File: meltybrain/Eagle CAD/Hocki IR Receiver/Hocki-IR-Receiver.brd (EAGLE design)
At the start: 160 x 100 mm, 0 parts

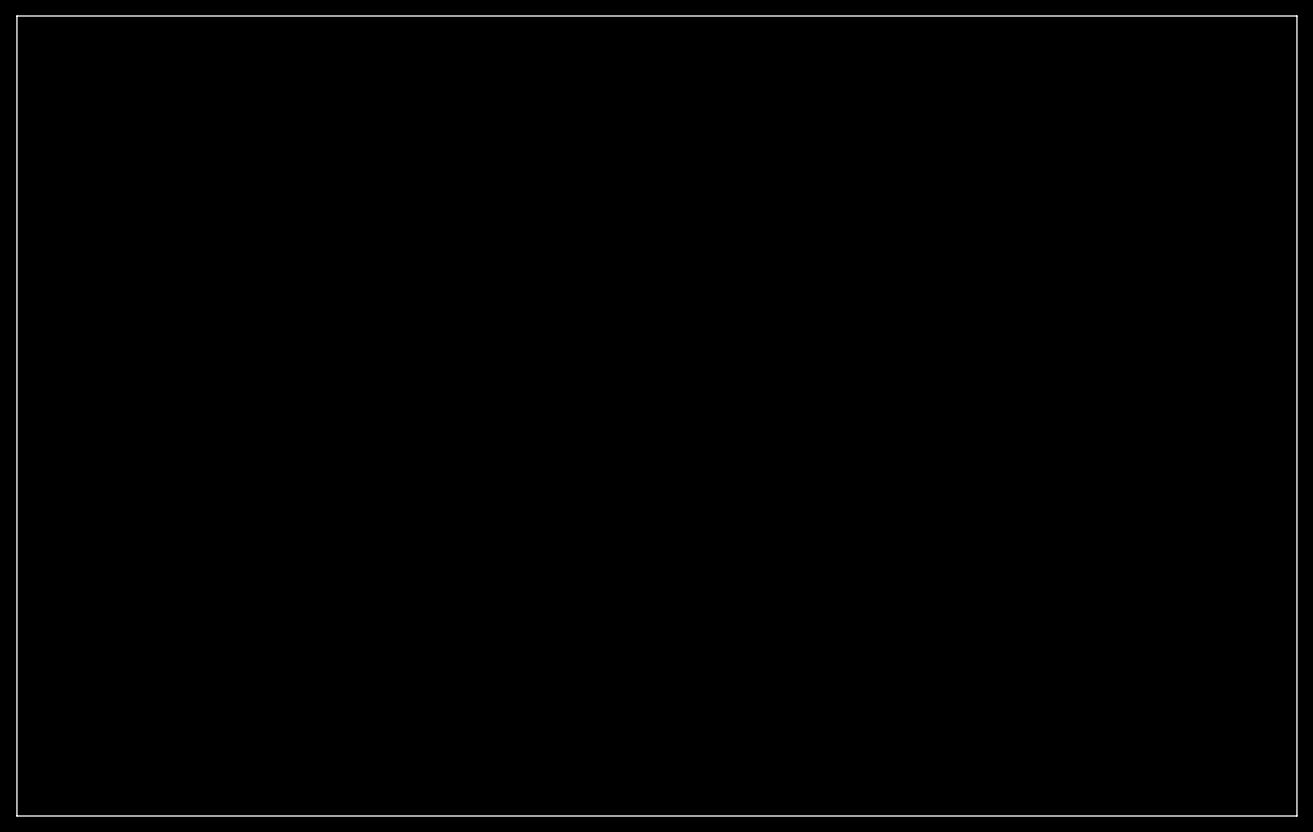
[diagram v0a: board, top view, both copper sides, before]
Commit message: broke something. this is a test
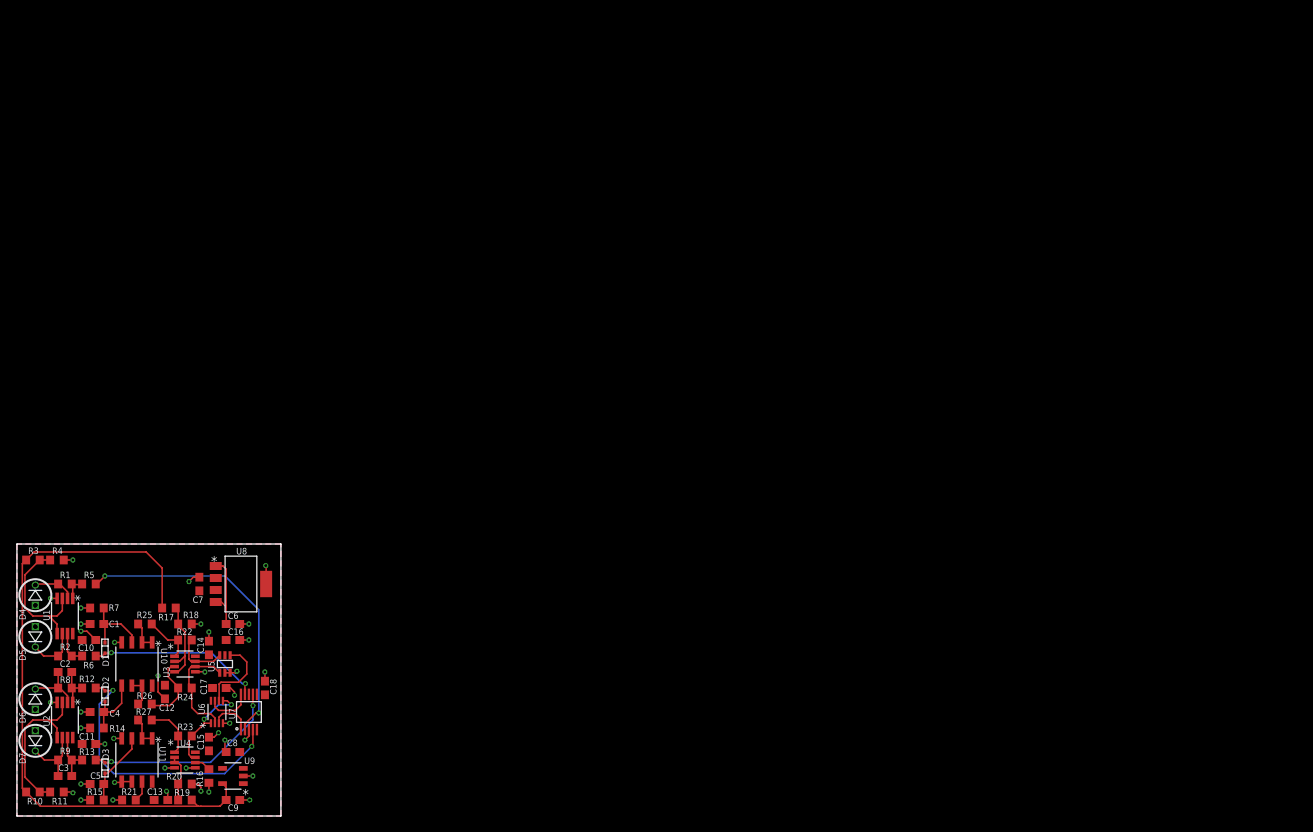
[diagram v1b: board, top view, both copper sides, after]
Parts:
- added C1, C4, C5: 50n, rcl:C0603
- added C10, C11, C6, C7, C8, C9: 1u, rcl:C0603
- added C12, C13, C14, C15, C16, C17, C18: 0.1u, rcl:C0603
- added C2: 0.5p, rcl:C0603
- added C3: 2p, rcl:C0603
- added D1, D2, D3: RB521S30T1G, Hocki_library:SOD-523
- added D4, D5, D6, D7: TEFD4300F, Hocki_library:TEFD4300F
- added R1: 10M, resistor:R0603
- added R10, R11, R16, R18, R20, R21, R22, R23, R24, R3, R4, R9: 10k, resistor:R0603
- added R12, R13, R5, R6: 50, resistor:R0603
- added R14, R15, R7: 30k, resistor:R0603
- added R17, R19: 3.33k, resistor:R0603
- added R2: 1M, resistor:R0603
- added R25, R26, R27: 30, resistor:R0603
- added R8: 100k, resistor:R0603
- added U1, U2: OPA2380AIDGKR, Hocki_library:8-VSSOP
- added U10, U11: LMH6612MAX/NOPB, Hocki_library:8-SOIC
- added U3, U4: TLV3502AIDCNR, Hocki_library:SOT-23-8
- added U5: SN74LVC1G58DCKR, Hocki_library:SC-70-6
- added U6: NL27WZ32USG, Hocki_library:US8
- added U7: TMUX1204DGSR, Hocki_library:10-VSSOP
- added U8: LP38693MP-5.0/NOPB, Hocki_library:SOT-223-5
- added U9: TLV73310PDBVT, Hocki_library:SOT-23-5
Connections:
- new net 1.0V: C9.1, R10.2, R17.2, R19.2, R3.2, U9.5
- new net 100KGAIN: D2.2, R12.2, U7.4
- new net 100KLOGIC: R24.1, U3.6, U5.1, U6.2
- new net 100KPEAK: C4.1, D2.1, R14.2, U10.5
- new net 10KGAIN: D3.2, R13.2, U7.7
- new net 10KLOGIC: R23.1, U4.7, U6.1, U6.5
- new net 10KPEAK: C5.1, D3.1, R15.2, U11.3
- new net 10MGAIN: R5.2, U7.2
- new net 1MGAIN: D1.2, R6.2, U7.9
- new net 1MLOGIC: R22.1, U3.7, U5.6
- new net 5V: C10.1, C11.1, C12.1, C13.1, C14.1, C15.1, C16.1, C17.1, C18.1, C7.1, C8.1, U1.8, U10.8, U11.8, U2.8, U3.8, U4.8, U5.5, U6.8, U7.5, U7.6, U8.3, U9.1, U9.3
- new net A0: U6.3, U7.1
- new net A1: U6.7, U7.10
- new net GND: C1.2, C10.2, C11.2, C12.2, C13.2, C14.2, C15.2, C16.2, C17.2, C18.2, C4.2, C5.2, C6.2, C7.2, C8.2, C9.2, D4.1, D5.1, D6.1, D7.1, R11.1, R14.1, R15.1, R16.1, R18.1, R20.1, R21.1, R4.1, R7.1, U1.4, U10.4, U11.4, U11.5, U11.6, U2.4, U3.5, U4.4, U4.5, U5.2, U5.3, U6.4, U7.3, U8.5, U9.2
- new net N$1: D4.2, R1.1, U1.2
- new net N$10: C3.1, D7.2, R9.1, U2.6
- new net N$11: C3.2, R13.1, R9.2, U2.7
- new net N$12: R10.1, R11.2, U2.3, U2.5
- new net N$13: R17.1, R18.2, U3.2, U3.4
- new net N$14: R19.1, R20.2, U4.2, U4.3
- new net N$15: R27.1, U11.1, U11.2
- new net N$16: R25.1, U10.1, U10.2
- new net N$17: C1.1, D1.1, R7.2, U10.3
- new net N$18: R26.1, U10.6, U10.7
- new net N$19: R21.2, U11.7
- new net N$2: R1.2, R5.1, U1.1
- new net N$20: R24.2, R26.2, U3.3
- new net N$22: R23.2, R27.2, U4.1
- new net N$23: R22.2, R25.2, U3.1
- new net N$3: D5.2, R2.1, U1.6
- new net N$4: R2.2, R6.1, U1.7
- new net N$5: R3.1, R4.2, U1.3, U1.5
- new net N$6: C2.1, D6.2, R8.1, U2.2
- new net N$7: R16.2, U4.6
- new net N$8: C2.2, R12.1, R8.2, U2.1
- new net N$9: U5.4, U6.6
- new net VG_SIGNAL: U7.8
- new net VIN: C6.1, U8.1, U8.4
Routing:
- net 1.0V: track 0.00 -> 82.0 mm
- net GND: track 0.00 -> 51.6 mm, vias 0 -> 38
- net 10MGAIN: track 0.00 -> 38.4 mm, vias 0 -> 2
- net 100KGAIN: track 0.00 -> 35.0 mm, vias 0 -> 2
- net 10KGAIN: track 0.00 -> 25.3 mm, vias 0 -> 2
- net 1MGAIN: track 0.00 -> 21.8 mm, vias 0 -> 2
- net N$12: track 0.00 -> 19.6 mm
- net N$5: track 0.00 -> 17.6 mm
- net 100KLOGIC: track 0.00 -> 13.3 mm
- net 10KLOGIC: track 0.00 -> 12.4 mm, vias 0 -> 2
- net N$13: track 0.00 -> 10.8 mm
- net N$9: track 0.00 -> 10.0 mm
- net VIN: track 0.00 -> 9.86 mm
- net N$17: track 0.00 -> 9.42 mm
- net 10KPEAK: track 0.00 -> 9.36 mm
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- added copper zone on layer 1, net 5V
- added copper zone on layer 16, net GND
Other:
- board size 160 x 100 mm -> 33 x 34 mm
